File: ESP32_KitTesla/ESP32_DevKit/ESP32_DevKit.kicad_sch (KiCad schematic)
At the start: 26 parts, among them J1 SM04B-SRSS-TB(LF)(SN), J2 Conn_01x19_Pin, J3 Conn_01x19_Pin, P1 USB_C_Plug, Q1 MMBT2222ALT1G, Q2 MMBT2222ALT1G, U1 AP2112K-3.3TRG1, U2 CH340C, U3 ESP32-WROVER-E

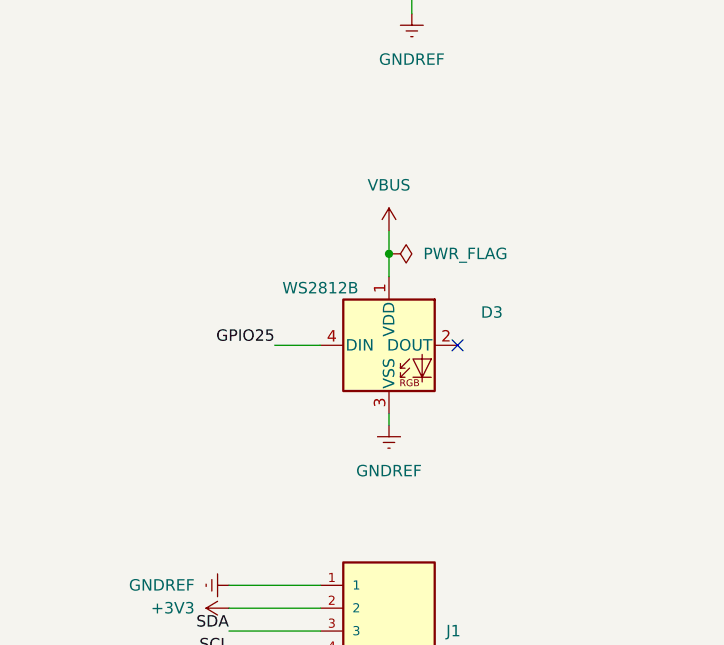
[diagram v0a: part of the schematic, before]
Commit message: ESP32_terminado
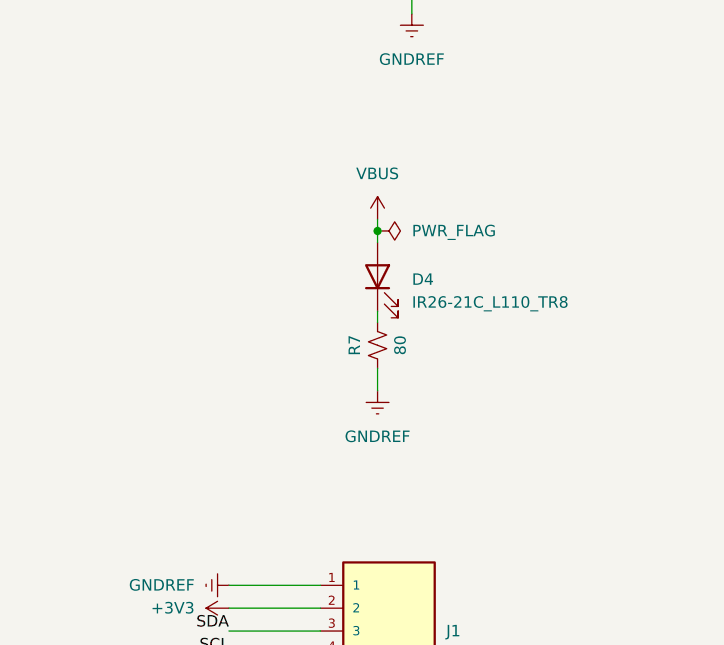
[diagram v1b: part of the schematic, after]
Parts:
- removed D3: WS2812B, LED_SMD:LED_WS2812B_PLCC4_5.0x5.0mm_P3.2mm, symbol LED:WS2812B
- added D4: IR26-21C_L110_TR8, LED_SMD:LED_1206_3216Metric_Pad1.42x1.75mm_HandSolder, symbol LED:IR26-21C_L110_TR8
- added R7: 80, Resistor_SMD:R_0805_2012Metric_Pad1.20x1.40mm_HandSolder, symbol Device:R_Small_US
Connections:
- net GNDREF: now also R7.2
- net VBUS: now also D4.2 (A)
- new net: D4.1 (K), R7.1
- no-connect marks 20 -> 19
